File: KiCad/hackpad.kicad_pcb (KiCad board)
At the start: 2 copper layers, 10 parts, among them SW1 RotaryEncoder_Switch, SW2 RotaryEncoder_Switch, SW3 RotaryEncoder_Switch, SW4 SW_Push, SW5 SW_Push, SW6 SW_Push, U1 Seeed Studio XIAO SAMD21, U2 PCF8574A

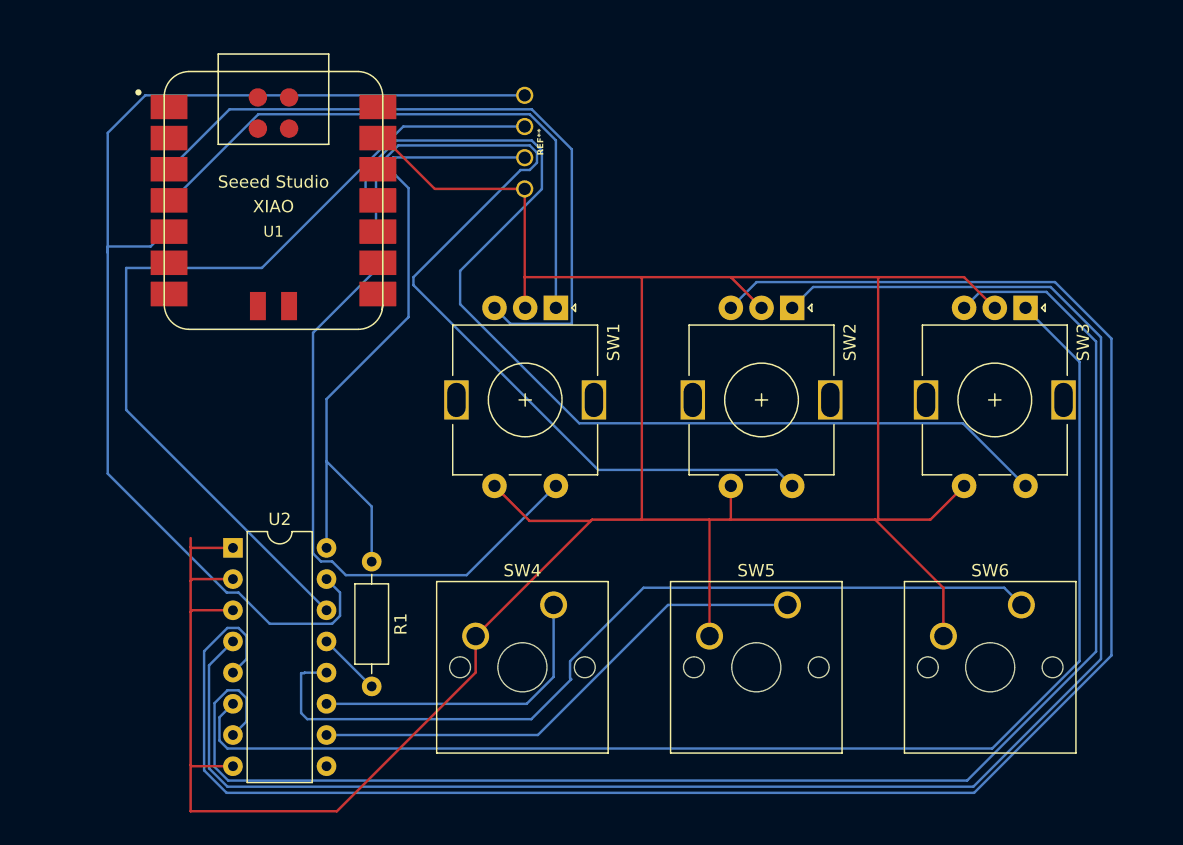
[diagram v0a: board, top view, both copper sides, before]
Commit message: HackPad Day 4 KiCad Files
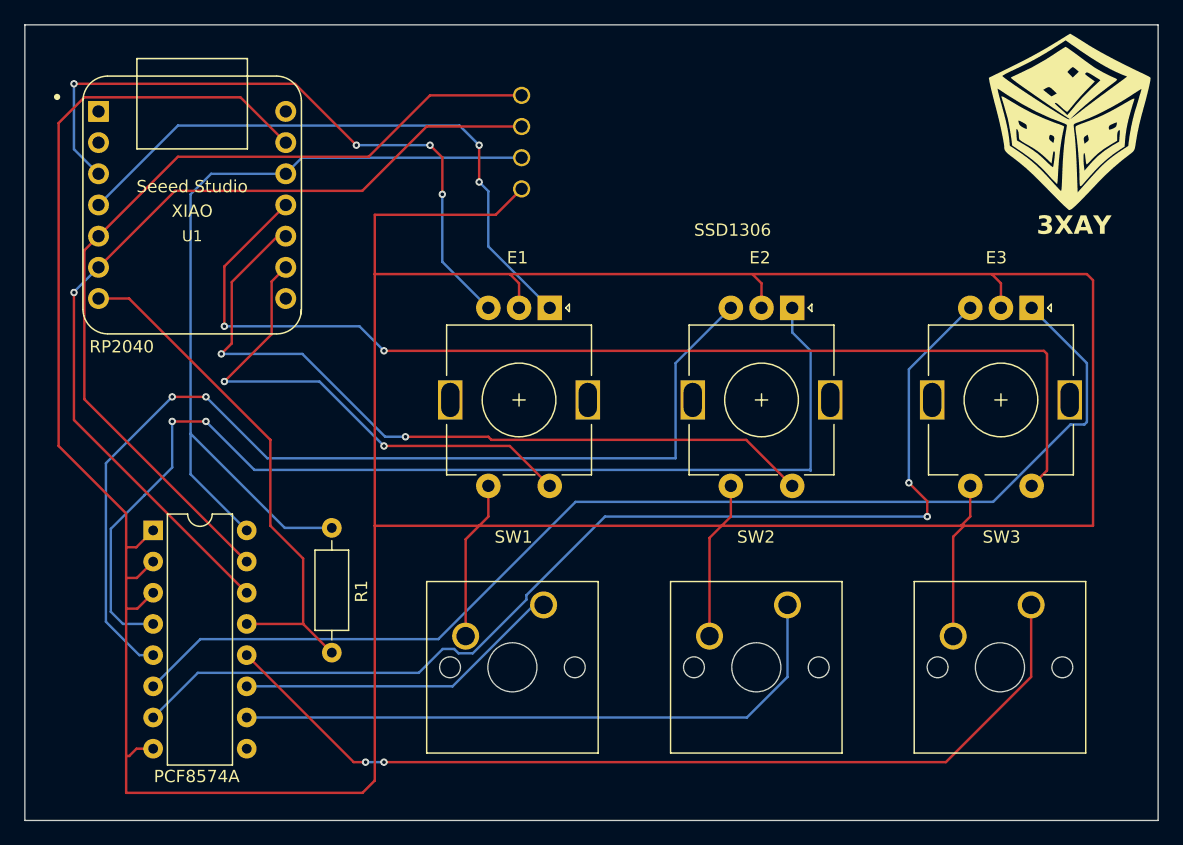
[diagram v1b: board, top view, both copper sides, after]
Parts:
- added G***: LOGO, LOGO, F.Cu at (200.8, 91.3)
- U1: footprint Seeed Studio XIAO Series Library:XIAO-SAMD21-RP2040-14P-2.54-21X17.8MM (Seeeduino XIAO) -> Seeed Studio XIAO Series Library:XIAO-Generic-Thruhole-14P-2.54-21X17.8MM
- moved U2 6.65 mm to (126.1, 124.7)
- moved U1 6.64 mm to (129.3, 98.2)
- moved R1 4.26 mm to (140.7, 124.5)
- moved SW4 0.81 mm to (157.9, 130.8)
- moved SW6 0.80 mm to (197.6, 130.8)
- moved SW1 0.50 mm to (158.4, 106.6)
- moved SW3 0.50 mm to (197.7, 106.6)
- moved OL1 0.25 mm to (156.1, 93.1)
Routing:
- net GND: track 250.7 -> 353.3 mm
- net Net-(U2-P1): track 156.5 -> 82.7 mm, vias 0 -> 2
- net Net-(U2-P0): track 142.5 -> 89.0 mm, vias 0 -> 2
- net IO_INT: track 5.20 -> 42.8 mm
- net Net-(U2-P3): track 126.8 -> 90.0 mm, vias 0 -> 2
- net Net-(OL1-SDA): track 96.8 -> 71.7 mm
- net VCC: track 56.1 -> 72.1 mm
- net Net-(U2-P2): track 107.3 -> 96.1 mm
- net Net-(U1-PA5_A9_D9_MISO): track 72.6 -> 63.1 mm, vias 0 -> 2
- net Net-(U2-P5): track 41.9 -> 51.3 mm
- net Net-(U1-PA7_A8_D8_SCK): track 49.3 -> 41.4 mm, vias 0 -> 2
- net Net-(U2-P7): track 70.2 -> 76.2 mm, vias 0 -> 2
- net Net-(U1-PA6_A10_D10_MOSI): track 85.8 -> 91.2 mm, vias 0 -> 2
- net Net-(U1-PA10_A2_D2): track 57.6 -> 54.4 mm, vias 0 -> 4
- net Net-(U2-P6): track 25.3 -> 26.9 mm
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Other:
- board outline added: 92.3 x 64.8 mm
- board text added: "3XAY"
- board text added: "E1"
- board text added: "E2"
- board text added: "E3"
- board text added: "PCF8574A"
- board text added: "R1"
- board text added: "RP2040"
- board text added: "SSD1306"
- board text added: "SW1"
- board text added: "SW2"
- board text added: "SW3"
